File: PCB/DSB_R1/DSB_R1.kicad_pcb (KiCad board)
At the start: 2 copper layers, 50.3 x 9.7 mm, 6 parts, among them J1 HEADER_2x05_PARALLEL, M1 HOLE, M2 HOLE, U1 DS18B20

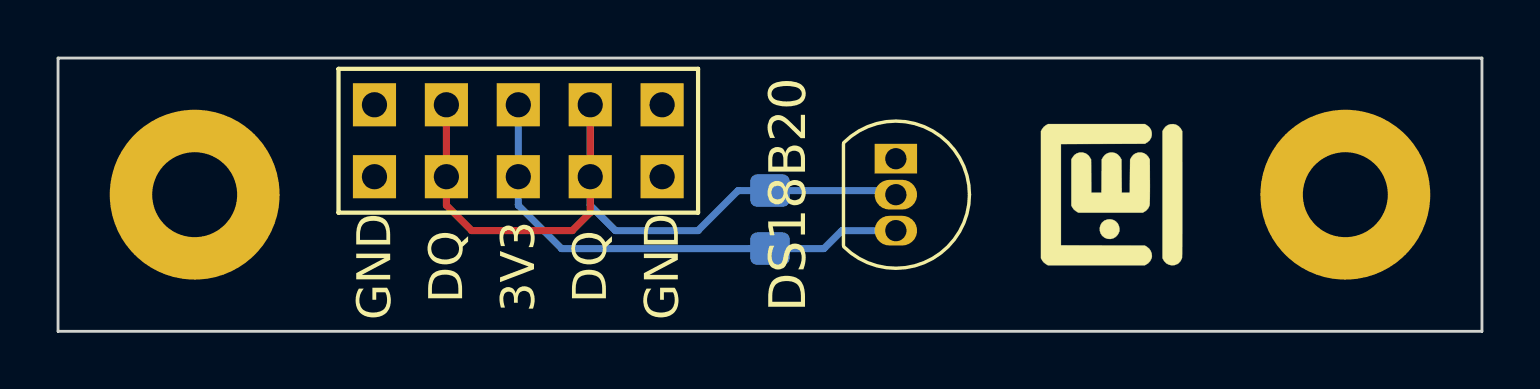
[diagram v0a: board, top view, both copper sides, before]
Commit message: rename and update
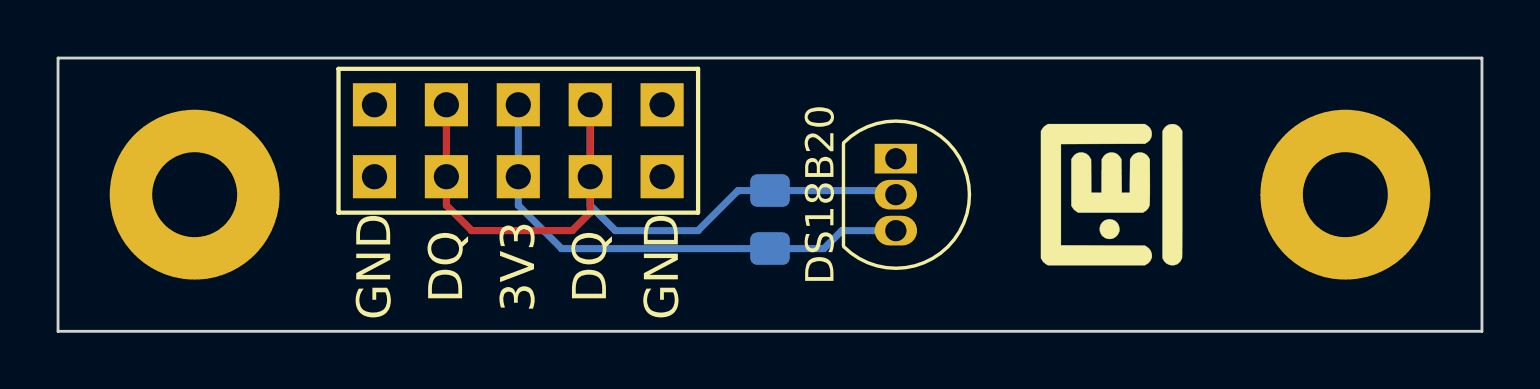
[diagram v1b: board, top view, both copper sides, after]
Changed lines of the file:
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@@
   (page A4)
   (layers
-    (0 F.Cu signal hide)
-    (31 B.Cu signal hide)
+    (0 F.Cu signal)
+    (31 B.Cu signal)
     (32 B.Adhes user)
     (33 F.Adhes user)
     (34 B.Paste user)
     (35 F.Paste user)
-    (36 B.SilkS user hide)
+    (36 B.SilkS user)
     (37 F.SilkS user)
     (38 B.Mask user)
-    (39 F.Mask user hide)
+    (39 F.Mask user)
     (40 Dwgs.User user)
     (41 Cmts.User user)
@@
     (44 Edge.Cuts user)
     (45 Margin user)
-    (46 B.CrtYd user hide)
+    (46 B.CrtYd user)
     (47 F.CrtYd user)
-    (48 B.Fab user hide)
-    (49 F.Fab user hide)
+    (48 B.Fab user)
+    (49 F.Fab user)
   )
   (setup
@@
       (usegerberattributes false)
       (usegerberadvancedattributes false)
-      (creategerberjobfile false)
+      (creategerberjobfile true)
       (excludeedgelayer true)
       (linewidth 0.100000)
@@
       (outputformat 1)
       (mirror false)
-      (drillshape 1)
+      (drillshape 0)
       (scaleselection 1)
-      (outputdirectory ""))
+      (outputdirectory "gerber/"))
   )
   (net 0 "")
@@
     )
   )
-  (gr_text DS18B20 (at 153.035 101.6 90) (layer F.SilkS)
-    (effects (font (size 1.3 1.3) (thickness 0.3)))
+  (gr_text DS18B20 (at 154.178 101.6 90) (layer F.SilkS)
+    (effects (font (size 1 1) (thickness 0.1)))
   )
   (gr_text DQ (at 146.05 104.14 90) (layer F.SilkS)
